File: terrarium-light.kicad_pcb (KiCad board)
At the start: 2 copper layers, 100 x 100 mm, 51 parts, among them J2 USB_C_Receptacle_USB2.0_16P, Q1 UMH3N, U1 CH340C, U2 TPS61169DCKR, U3 TPS61169DCKR, U4 LM1117S-3.3, U6 ESP32-S3-MINI-1

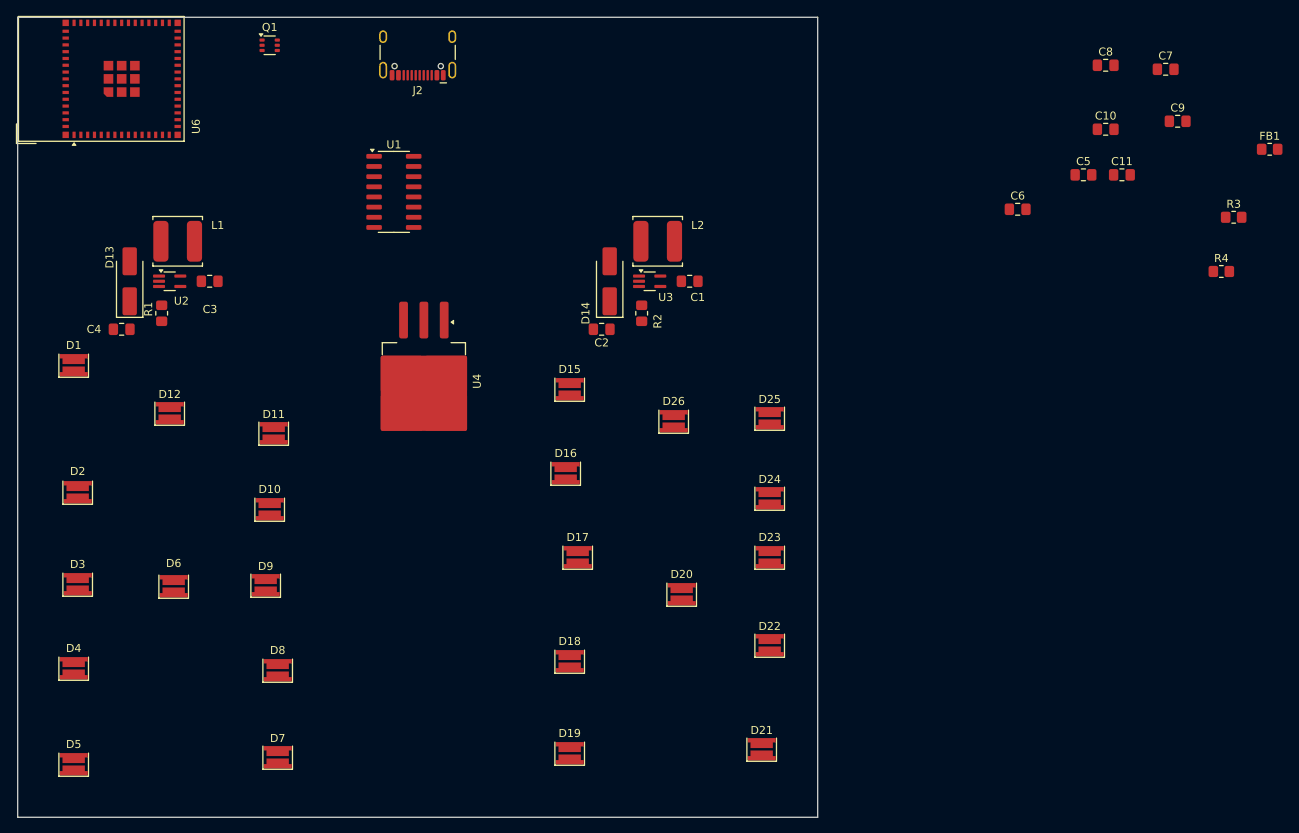
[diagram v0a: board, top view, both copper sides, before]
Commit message: more layout
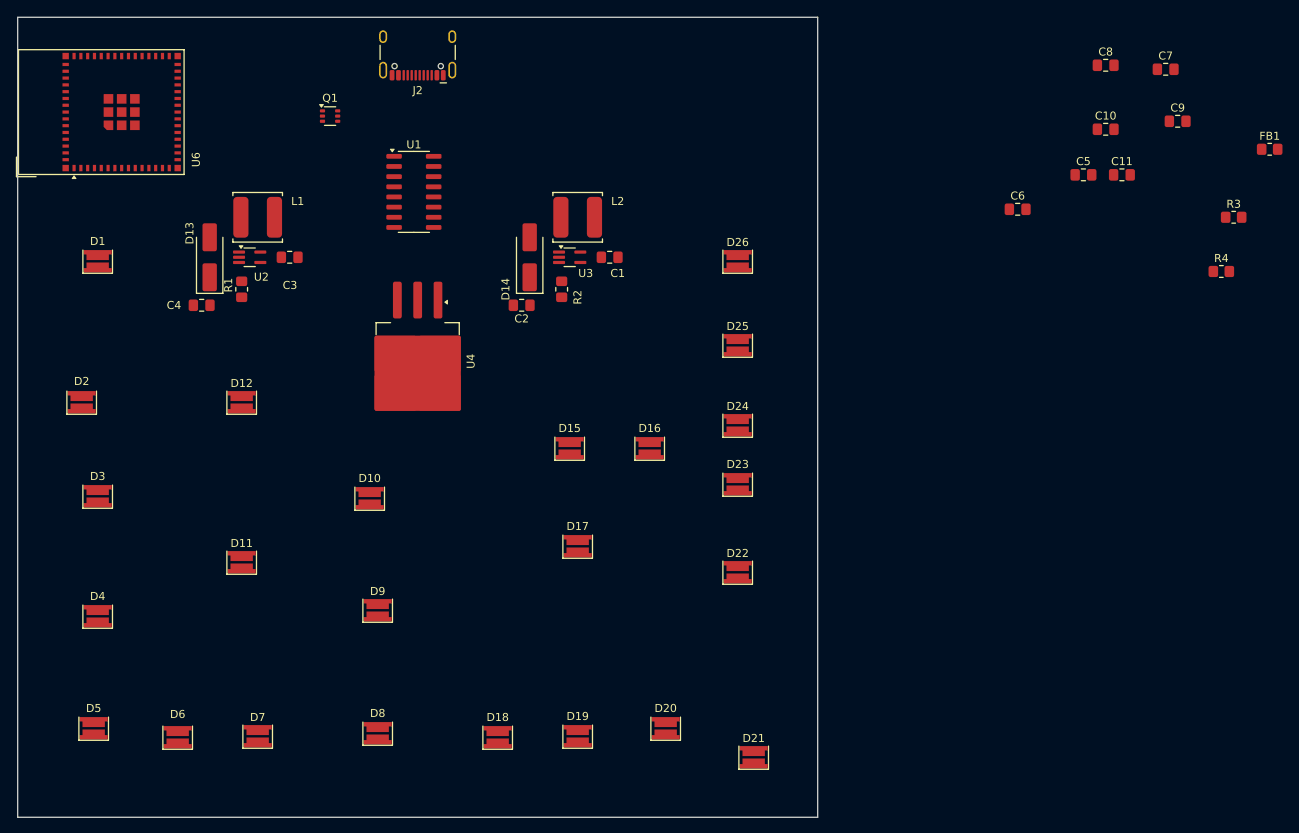
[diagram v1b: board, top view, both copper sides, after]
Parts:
- moved D26 21.5 mm to (140.0, 80.5)
- moved D6 18.9 mm to (70.0, 140.0)
- moved D20 16.9 mm to (131.0, 138.9)
- moved D11 16.6 mm to (78.0, 118.1)
- moved D8 14.8 mm to (95.0, 139.5)
- moved D9 14.3 mm to (95.0, 124.1)
- moved D1 13.3 mm to (60.0, 80.5)
- moved D18 13.1 mm to (110.0, 140.0)
- moved D10 12.6 mm to (94.0, 110.1)
- moved Q1 11.6 mm to (89.0, 62.4)
- moved D3 11.3 mm to (60.0, 109.9)
- moved D2 11.3 mm to (58.0, 98.1)
- moved D16 11.0 mm to (129.0, 103.9)
- moved C1 10.4 mm to (124.0, 80.0)
- moved C2 10.4 mm to (113.0, 86.0)
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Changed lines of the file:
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@@
 	(footprint "Resistor_SMD:R_0805_2012Metric_Pad1.20x1.40mm_HandSolder"
 		(layer "F.Cu")
-		(at 68 87 -90)
+		(at 78 84 -90)
 		(descr "Resistor SMD 0805 (2012 Metric), square (rectangular) end terminal, IPC_7351 nominal with elongated pad for handsoldering. (Body size source: IPC-SM-782 page 72, https://www.pcb-3d.com/wordpress/wp-content/uploads/ipc-sm-782a_amendment_1_and_2.pdf), generated with kicad-footprint-generator")
 		(tags "resistor handsolder")
@@
 	(footprint "LED_SMD:LED_SPMWHD32AMH0XAR0PR"
 		(layer "F.Cu")
-		(at 119 130.5)
+		(at 110 140)
 		(property "Reference" "D18"
 			(at 0 -2.5 0)
@@
 	(footprint "LED_SMD:LED_SPMWHD32AMH0XAR0PR"
 		(layer "F.Cu")
-		(at 82.5 131.625)
+		(at 95 139.5)
 		(property "Reference" "D8"
 			(at 0 -2.5 0)
@@
 	(footprint "Package_TO_SOT_SMD:SOT-363_SC-70-6"
 		(layer "F.Cu")
-		(at 81.5 53.5)
+		(at 89.05 62.35)
 		(descr "SOT-363, SC-70-6")
 		(tags "SOT-363 SC-70-6")
@@
 	(footprint "LED_SMD:LED_SPMWHD32AMH0XAR0PR"
 		(layer "F.Cu")
-		(at 57 131.375)
+		(at 60 124.875)
 		(property "Reference" "D4"
 			(at 0 -2.5 0)
@@
 	(footprint "LED_SMD:LED_SPMWHD32AMH0XAR0PR"
 		(layer "F.Cu")
-		(at 132 100.5)
+		(at 140 80.5)
 		(property "Reference" "D26"
-			(at 0 -2.5 0)
+			(at 0 -2.375 0)
 			(unlocked yes)
 			(layer "F.SilkS")
@@
 	(footprint "LED_SMD:LED_SPMWHD32AMH0XAR0PR"
 		(layer "F.Cu")
-		(at 69 99.5)
+		(at 78 98.125)
 		(property "Reference" "D12"
 			(at 0 -2.375 0)
@@
 	(footprint "Capacitor_SMD:C_0805_2012Metric_Pad1.18x1.45mm_HandSolder"
 		(layer "F.Cu")
-		(at 63 89 180)
+		(at 73 86 180)
 		(descr "Capacitor SMD 0805 (2012 Metric), square (rectangular) end terminal, IPC_7351 nominal with elongated pad for handsoldering. (Body size source: IPC-SM-782 page 76, https://www.pcb-3d.com/wordpress/wp-content/uploads/ipc-sm-782a_amendment_1_and_2.pdf, https://docs.google.com/spreadsheets/d/1BsfQQcO9C6DZCsRaXUlFlo91Tg2WpOkGARC1WS5S8t0/edit?usp=sharing), generated with kicad-footprint-generator")
 		(tags "capacitor handsolder")
@@
 	(footprint "LED_SMD:LED_SPMWHD32AMH0XAR0PR"
 		(layer "F.Cu")
-		(at 119 96.5)
+		(at 119 103.875)
 		(property "Reference" "D15"
 			(at 0 -2.5 0)
@@
 	(footprint "LED_SMD:LED_SPMWHD32AMH0XAR0PR"
 		(layer "F.Cu")
-		(at 57.5 120.875)
+		(at 60 109.875)
 		(property "Reference" "D3"
 			(at 0 -2.5 0)
@@
 	(footprint "LED_SMD:LED_SPMWHD32AMH0XAR0PR"
 		(layer "F.Cu")
-		(at 120 117.5)
+		(at 120 116.125)
 		(property "Reference" "D17"
 			(at 0 -2.5 0)
@@
 	(footprint "Diode_SMD:D_SMA_Handsoldering"
 		(layer "F.Cu")
-		(at 124 83 90)
+		(at 114 80 90)
 		(descr "Diode SMA (DO-214AC) Handsoldering")
 		(tags "Diode SMA (DO-214AC) Handsoldering")
@@
 	(footprint "LED_SMD:LED_SPMWHD32AMH0XAR0PR"
 		(layer "F.Cu")
-		(at 57 93.5)
+		(at 60 80.5)
 		(property "Reference" "D1"
 			(at 0 -2.5 0)
@@
 	(footprint "Package_SO:SOIC-16_3.9x9.9mm_P1.27mm"
 		(layer "F.Cu")
-		(at 97.025 71.825)
+		(at 99.525 71.825)
 		(descr "SOIC, 16 Pin (JEDEC MS-012AC, https://www.analog.com/media/en/package-pcb-resources/package/pkg_pdf/soic_narrow-r/r_16.pdf), generated with kicad-footprint-generator ipc_gullwing_generator.py")
 		(tags "SOIC SO")
@@
 	(footprint "Inductor_SMD:L_TDK_VLS6045EX_VLS6045AF"
 		(layer "F.Cu")
-		(at 70 78 180)
+		(at 80 75 180)
 		(descr "Inductor,TDK, VLS-6045, 6x6x4.5mm, https://product.tdk.com/system/files/dam/doc/product/inductor/inductor/smd/catalog/inductor_commercial_power_vls6045ex_en.pdf")
 		(tags "inductor TDK VLS SMD VLS6045EF VLS6045AF")
@@
 	(footprint "Capacitor_SMD:C_0805_2012Metric_Pad1.18x1.45mm_HandSolder"
 		(layer "F.Cu")
-		(at 123 89 180)
+		(at 113 86 180)
 		(descr "Capacitor SMD 0805 (2012 Metric), square (rectangular) end terminal, IPC_7351 nominal with elongated pad for handsoldering. (Body size source: IPC-SM-782 page 76, https://www.pcb-3d.com/wordpress/wp-content/uploads/ipc-sm-782a_amendment_1_and_2.pdf, https://docs.google.com/spreadsheets/d/1BsfQQcO9C6DZCsRaXUlFlo91Tg2WpOkGARC1WS5S8t0/edit?usp=sharing), generated with kicad-footprint-generator")
 		(tags "capacitor handsolder")
@@
 	(footprint "Package_TO_SOT_SMD:SOT-353_SC-70-5_Handsoldering"
 		(layer "F.Cu")
-		(at 69 83)
+		(at 79 80)
 		(descr "SOT-353, SC-70-5, Handsoldering")
 		(tags "SOT-353 SC-70-5 Handsoldering")
@@
 	(footprint "LED_SMD:LED_SPMWHD32AMH0XAR0PR"
 		(layer "F.Cu")
-		(at 144 100.125)
+		(at 140 91)
 		(property "Reference" "D25"
 			(at 0 -2.375 0)
@@
 	(footprint "LED_SMD:LED_SPMWHD32AMH0XAR0PR"
 		(layer "F.Cu")
-		(at 82.5 142.5)
+		(at 80 139.875)
 		(property "Reference" "D7"
 			(at 0 -2.375 0)
@@
 	(footprint "Diode_SMD:D_SMA_Handsoldering"
 		(layer "F.Cu")
-		(at 64 83 90)
+		(at 74 80 90)
 		(descr "Diode SMA (DO-214AC) Handsoldering")
 		(tags "Diode SMA (DO-214AC) Handsoldering")
@@
 	(footprint "RF_Module:ESP32-S2-MINI-1"
 		(layer "F.Cu")
-		(at 60.45 57.7 90)
+		(at 60.45 61.85 90)
 		(descr "2.4 GHz Wi-Fi and Bluetooth combo chip, external antenna, https://www.espressif.com/sites/default/files/documentation/esp32-s3-mini-1_mini-1u_datasheet_en.pdf")
 		(tags "2.4 GHz Wi-Fi Bluetooth external antenna espressif  20*15.4mm")
@@
 			(polygon
 				(pts
-					(xy 55.2 35) (xy 55.2 80.4) (xy 35.7 80.4) (xy 35.7 35)
+					(xy 55.2 39.15) (xy 55.2 84.55) (xy 35.7 84.55) (xy 35.7 39.15)
 				)
 			)
@@
 	(footprint "LED_SMD:LED_SPMWHD32AMH0XAR0PR"
 		(layer "F.Cu")
-		(at 81.5 111.5)
+		(at 94 110.125)
 		(property "Reference" "D10"
 			(at 0 -2.5 0)
@@
 	(footprint "LED_SMD:LED_SPMWHD32AMH0XAR0PR"
 		(layer "F.Cu")
-		(at 57.5 109.375)
+		(at 58 98.125)
 		(property "Reference" "D2"
 			(at 0 -2.625 0)
@@
 	(footprint "LED_SMD:LED_SPMWHD32AMH0XAR0PR"
 		(layer "F.Cu")
-		(at 133 122.125)
+		(at 131 138.875)
 		(property "Reference" "D20"
 			(at 0 -2.5 0)
@@
 	(footprint "LED_SMD:LED_SPMWHD32AMH0XAR0PR"
 		(layer "F.Cu")
-		(at 81 121)
+		(at 95 124.125)
 		(property "Reference" "D9"
 			(at 0 -2.375 0)
@@
 	(footprint "Inductor_SMD:L_TDK_VLS6045EX_VLS6045AF"
 		(layer "F.Cu")
-		(at 130 78 180)
+		(at 120 75 180)
 		(descr "Inductor,TDK, VLS-6045, 6x6x4.5mm, https://product.tdk.com/system/files/dam/doc/product/inductor/inductor/smd/catalog/inductor_commercial_power_vls6045ex_en.pdf")
 		(tags "inductor TDK VLS SMD VLS6045EF VLS6045AF")
@@
 	(footprint "Capacitor_SMD:C_0805_2012Metric_Pad1.18x1.45mm_HandSolder"
 		(layer "F.Cu")
-		(at 134 83)
+		(at 124 80)
 		(descr "Capacitor SMD 0805 (2012 Metric), square (rectangular) end terminal, IPC_7351 nominal with elongated pad for handsoldering. (Body size source: IPC-SM-782 page 76, https://www.pcb-3d.com/wordpress/wp-content/uploads/ipc-sm-782a_amendment_1_and_2.pdf, https://docs.google.com/spreadsheets/d/1BsfQQcO9C6DZCsRaXUlFlo91Tg2WpOkGARC1WS5S8t0/edit?usp=sharing), generated with kicad-footprint-generator")
 		(tags "capacitor handsolder")
@@
 	(footprint "LED_SMD:LED_SPMWHD32AMH0XAR0PR"
 		(layer "F.Cu")
-		(at 143 141.5)
+		(at 142 142.5)
 		(property "Reference" "D21"
 			(at 0 -2.375 0)
@@
 	(footprint "Resistor_SMD:R_0805_2012Metric_Pad1.20x1.40mm_HandSolder"
 		(layer "F.Cu")
-		(at 128 87 -90)
+		(at 118 84 -90)
 		(descr "Resistor SMD 0805 (2012 Metric), square (rectangular) end terminal, IPC_7351 nominal with elongated pad for handsoldering. (Body size source: IPC-SM-782 page 72, https://www.pcb-3d.com/wordpress/wp-content/uploads/ipc-sm-782a_amendment_1_and_2.pdf), generated with kicad-footprint-generator")
 		(tags "resistor handsolder")
@@
 	(footprint "LED_SMD:LED_SPMWHD32AMH0XAR0PR"
 		(layer "F.Cu")
-		(at 144 117.5)
+		(at 140 108.375)
 		(property "Reference" "D23"
 			(at 0 -2.5 0)
@@
 	(footprint "LED_SMD:LED_SPMWHD32AMH0XAR0PR"
 		(layer "F.Cu")
-		(at 118.5 107)
+		(at 129 103.875)
 		(property "Reference" "D16"
 			(at 0 -2.5 0)
@@
 	(footprint "LED_SMD:LED_SPMWHD32AMH0XAR0PR"
 		(layer "F.Cu")
-		(at 144 128.5)
+		(at 140 119.375)
 		(property "Reference" "D22"
 			(at 0 -2.375 0)
@@
 	(footprint "LED_SMD:LED_SPMWHD32AMH0XAR0PR"
 		(layer "F.Cu")
-		(at 69.5 121.125)
+		(at 70 140)
 		(property "Reference" "D6"
 			(at 0 -2.875 0)
@@
 	(footprint "LED_SMD:LED_SPMWHD32AMH0XAR0PR"
 		(layer "F.Cu")
-		(at 144 110.125)
+		(at 140 101)
 		(property "Reference" "D24"
 			(at 0 -2.375 0)
@@
 	(footprint "LED_SMD:LED_SPMWHD32AMH0XAR0PR"
 		(layer "F.Cu")
-		(at 57 143.375)
+		(at 59.5 138.875)
 		(property "Reference" "D5"
 			(at 0 -2.5 0)
@@
 	(footprint "Package_TO_SOT_SMD:SOT-353_SC-70-5_Handsoldering"
 		(layer "F.Cu")
-		(at 129 83)
+		(at 119 80)
 		(descr "SOT-353, SC-70-5, Handsoldering")
 		(tags "SOT-353 SC-70-5 Handsoldering")
@@
 	(footprint "LED_SMD:LED_SPMWHD32AMH0XAR0PR"
 		(layer "F.Cu")
-		(at 82 102)
+		(at 78 118.125)
 		(property "Reference" "D11"
 			(at 0 -2.375 0)
@@
 	(footprint "Package_TO_SOT_SMD:TO-263-3_TabPin2"
 		(layer "F.Cu")
-		(at 100.775 95.5 -90)
+		(at 100 93 -90)
 		(descr "TO-263/D2PAK/DDPAK SMD package, http://www.infineon.com/cms/en/product/packages/PG-TO263/PG-TO263-3-1/")
 		(tags "D2PAK DDPAK TO-263 D2PAK-3 TO-263-3 SOT-404")
@@
 	(footprint "Capacitor_SMD:C_0805_2012Metric_Pad1.18x1.45mm_HandSolder"
 		(layer "F.Cu")
-		(at 74 83)
+		(at 84 80)
 		(descr "Capacitor SMD 0805 (2012 Metric), square (rectangular) end terminal, IPC_7351 nominal with elongated pad for handsoldering. (Body size source: IPC-SM-782 page 76, https://www.pcb-3d.com/wordpress/wp-content/uploads/ipc-sm-782a_amendment_1_and_2.pdf, https://docs.google.com/spreadsheets/d/1BsfQQcO9C6DZCsRaXUlFlo91Tg2WpOkGARC1WS5S8t0/edit?usp=sharing), generated with kicad-footprint-generator")
 		(tags "capacitor handsolder")
@@
 	(footprint "LED_SMD:LED_SPMWHD32AMH0XAR0PR"
 		(layer "F.Cu")
-		(at 119 142)
+		(at 120 139.875)
 		(property "Reference" "D19"
 			(at 0 -2.5 0)
